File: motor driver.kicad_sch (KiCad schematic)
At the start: 6 parts, among them J1 Conn_01x04_Pin, J2 Screw_Terminal_01x02, J3 Screw_Terminal_01x02, J4 Screw_Terminal_01x02, U1 L293D, U2 L7805

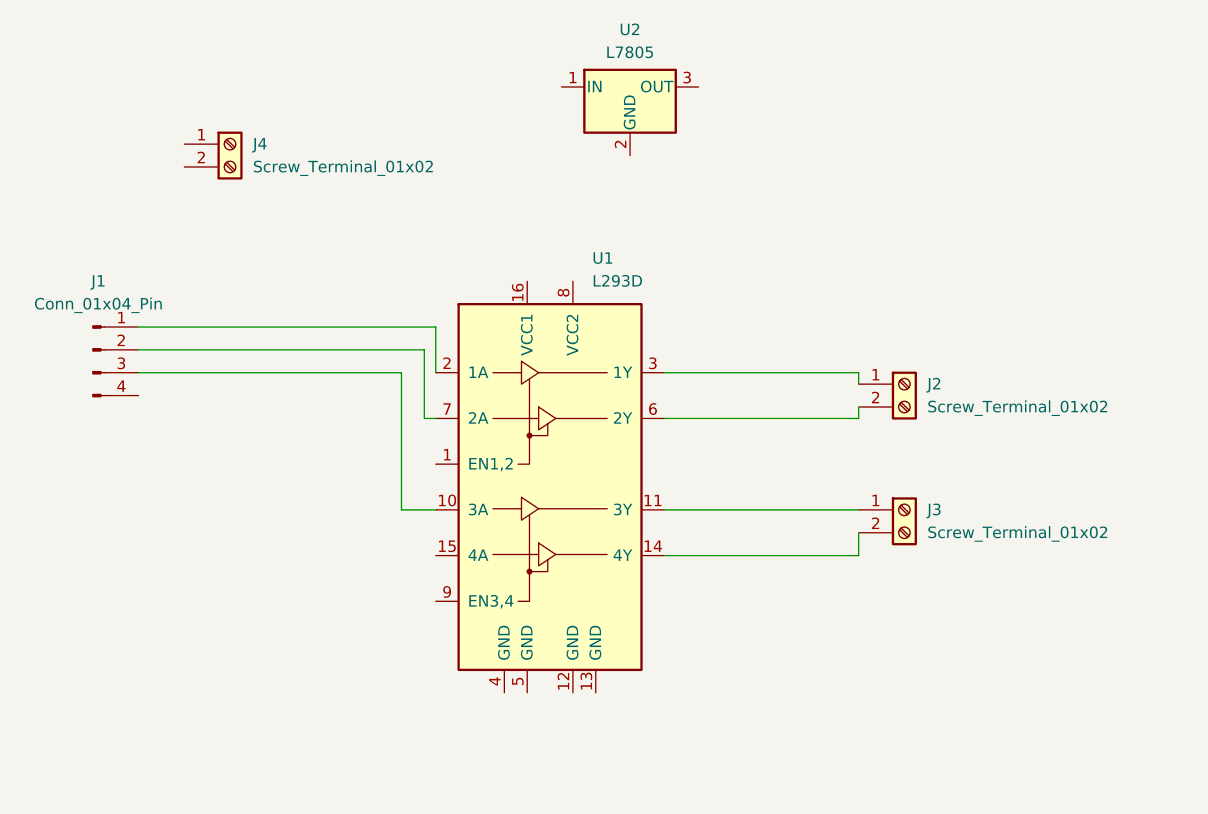
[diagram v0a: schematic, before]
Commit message: done
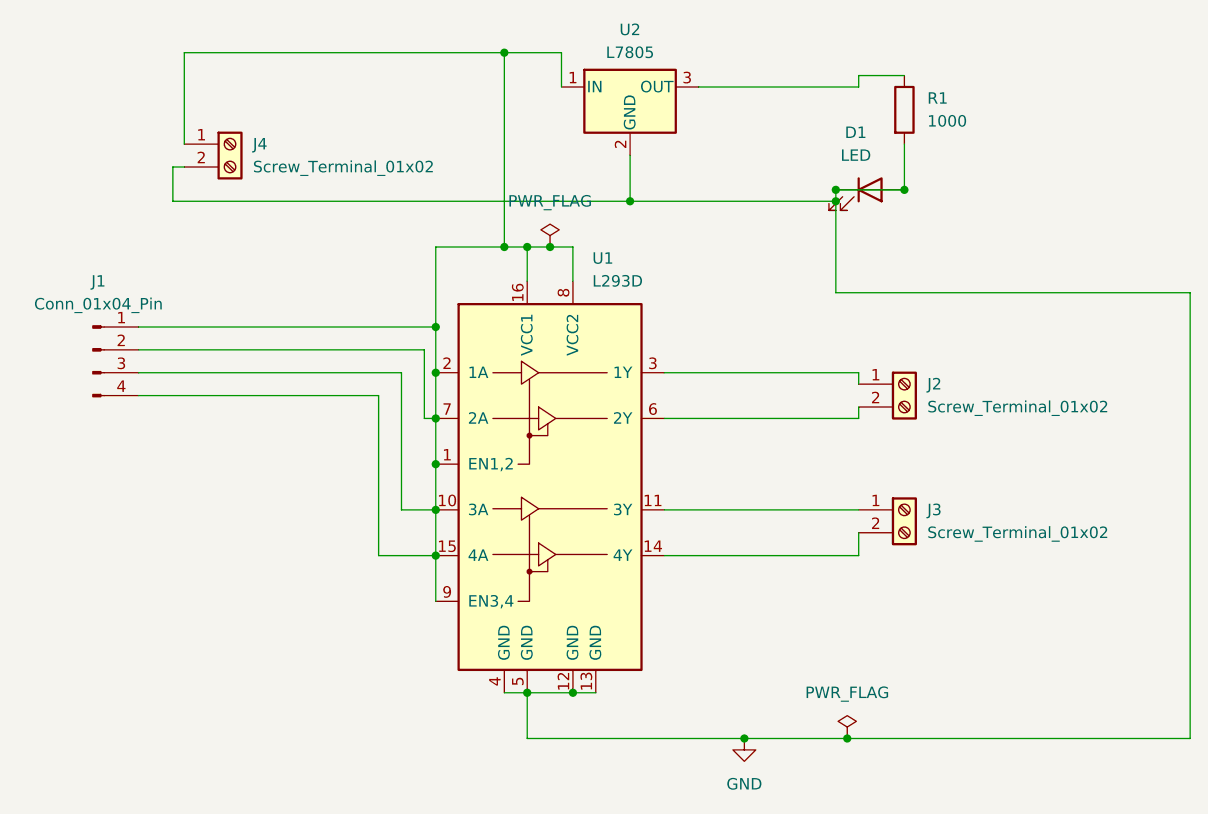
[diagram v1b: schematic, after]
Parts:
- added D1: LED, LED_THT:LED_VCCLite_5381H7_6.35x6.35mm, symbol Device:LED
- added R1: 1000, Resistor_THT:R_Axial_DIN0207_L6.3mm_D2.5mm_P15.24mm_Horizontal, symbol Device:R
- J1: footprint (none) -> Connector_Molex:Molex_KK-254_AE-6410-04A_1x04_P2.54mm_Vertical
- J2, J3, J4: footprint (none) -> TerminalBlock_Phoenix:TerminalBlock_Phoenix_MKDS-1,5-2_1x02_P5.00mm_Horizontal
- U2: footprint (none) -> Package_TO_SOT_SMD:TO-252-3_TabPin2
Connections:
- net at J1.1 (Pin_1), U1.2 (1A): now also J1.2 (Pin_2), J1.3 (Pin_3), J1.4 (Pin_4), J4.1 (Pin_1), U1.1 (EN1,2), U1.10 (3A), U1.15 (4A), U1.16 (VCC1), U1.7 (2A), U1.8 (VCC2), U1.9 (EN3,4), U2.1 (IN)
- net GND: now reaches J4.2 (Pin_2)
- net GND: now also U1.12 (GND), U1.13 (GND), U1.4 (GND), U1.5 (GND), U2.2 (GND), D1.1 (K), D1.2 (A), R1.2
- net at U2.3 (OUT): now also R1.1
